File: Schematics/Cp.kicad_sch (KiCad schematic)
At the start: 55 parts, among them Q10 J201, Q11 J201, Q3 2SC1815, Q4 2SC1815, Q5 2SC1815, Q6 2SC1815, Q7 2SC1815, Q8 2SC1815, SW1 SW_SPDT, U1 CA3080

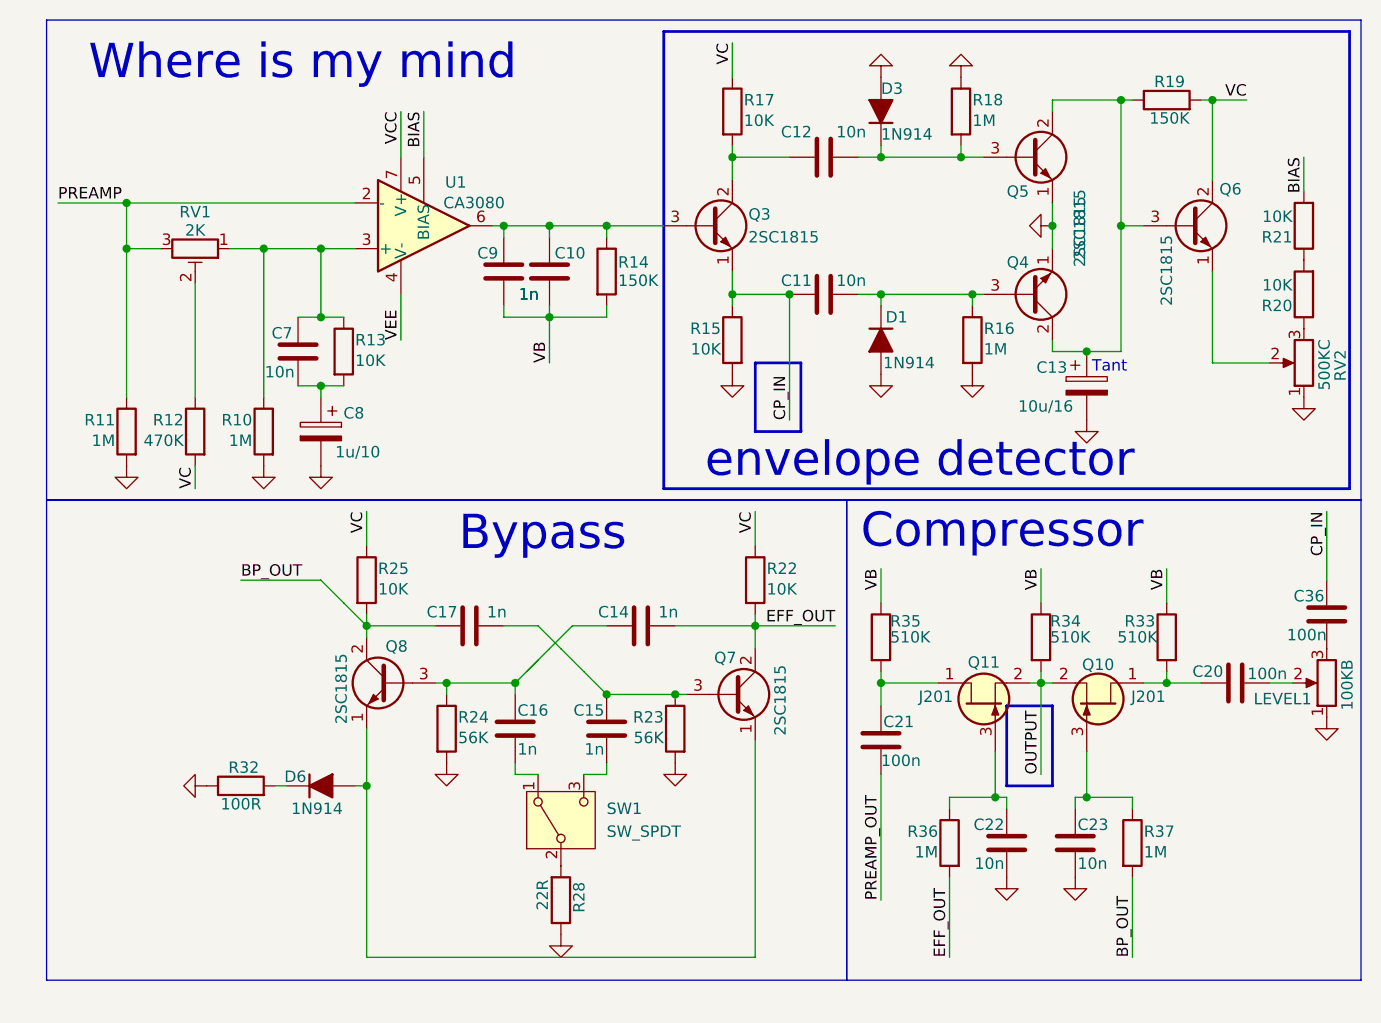
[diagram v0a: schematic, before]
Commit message: smal schem upd
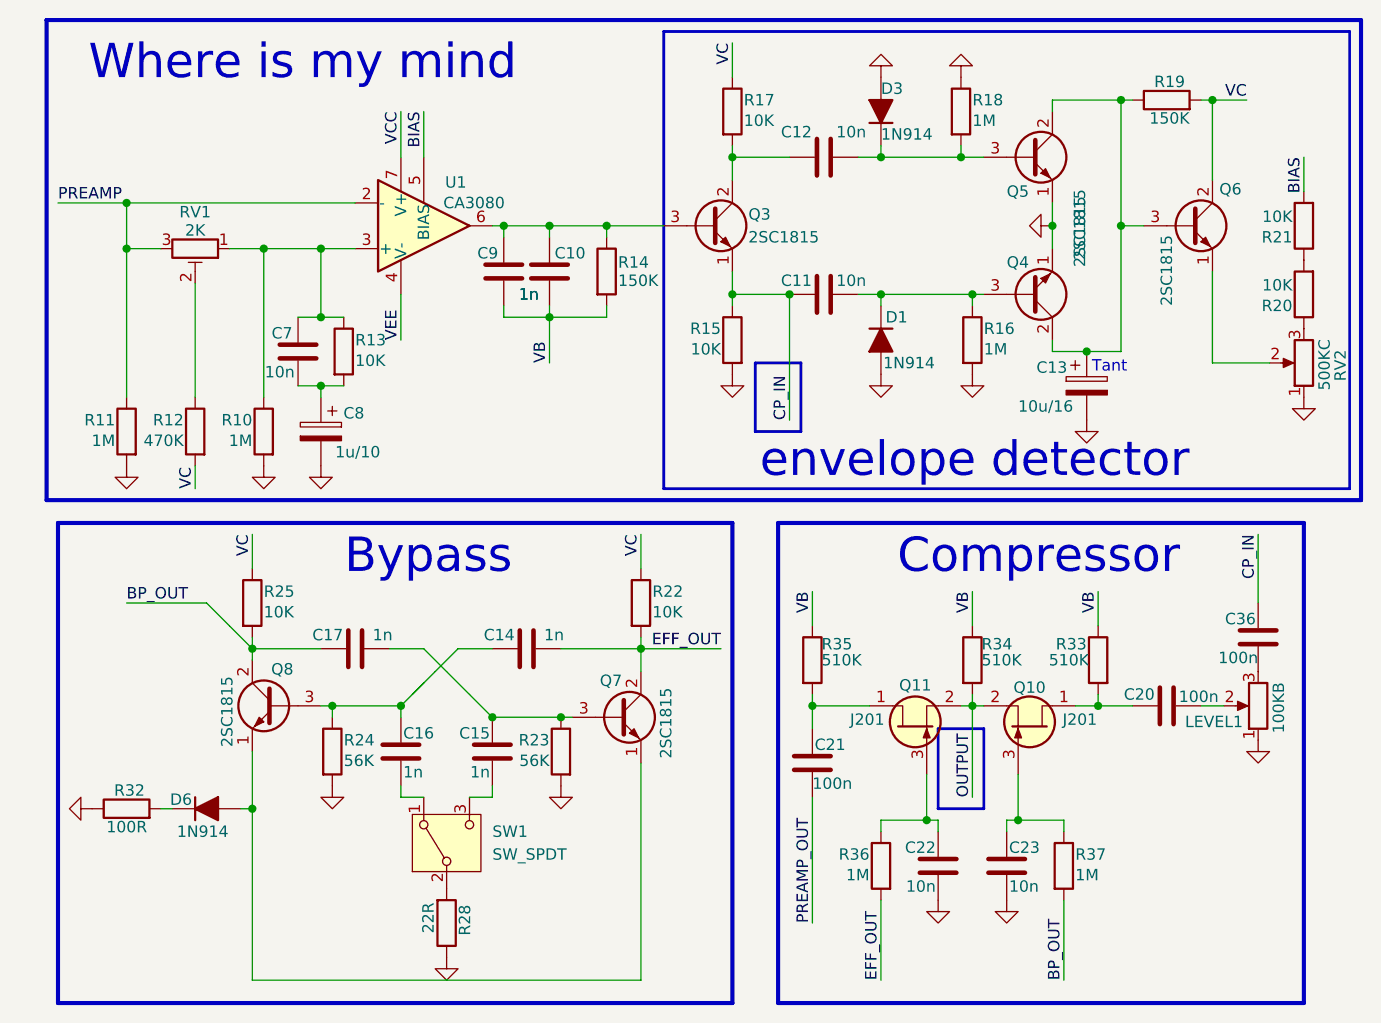
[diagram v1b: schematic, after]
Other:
- moved on the sheet: C14, C15, C16, C17, C20, C21, C22, C23, C36, D6, LEVEL1, Q10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
